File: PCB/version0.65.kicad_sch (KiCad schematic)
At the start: 142 parts, among them SW1 SW_SPDT, U1 SuperMini nRF52840

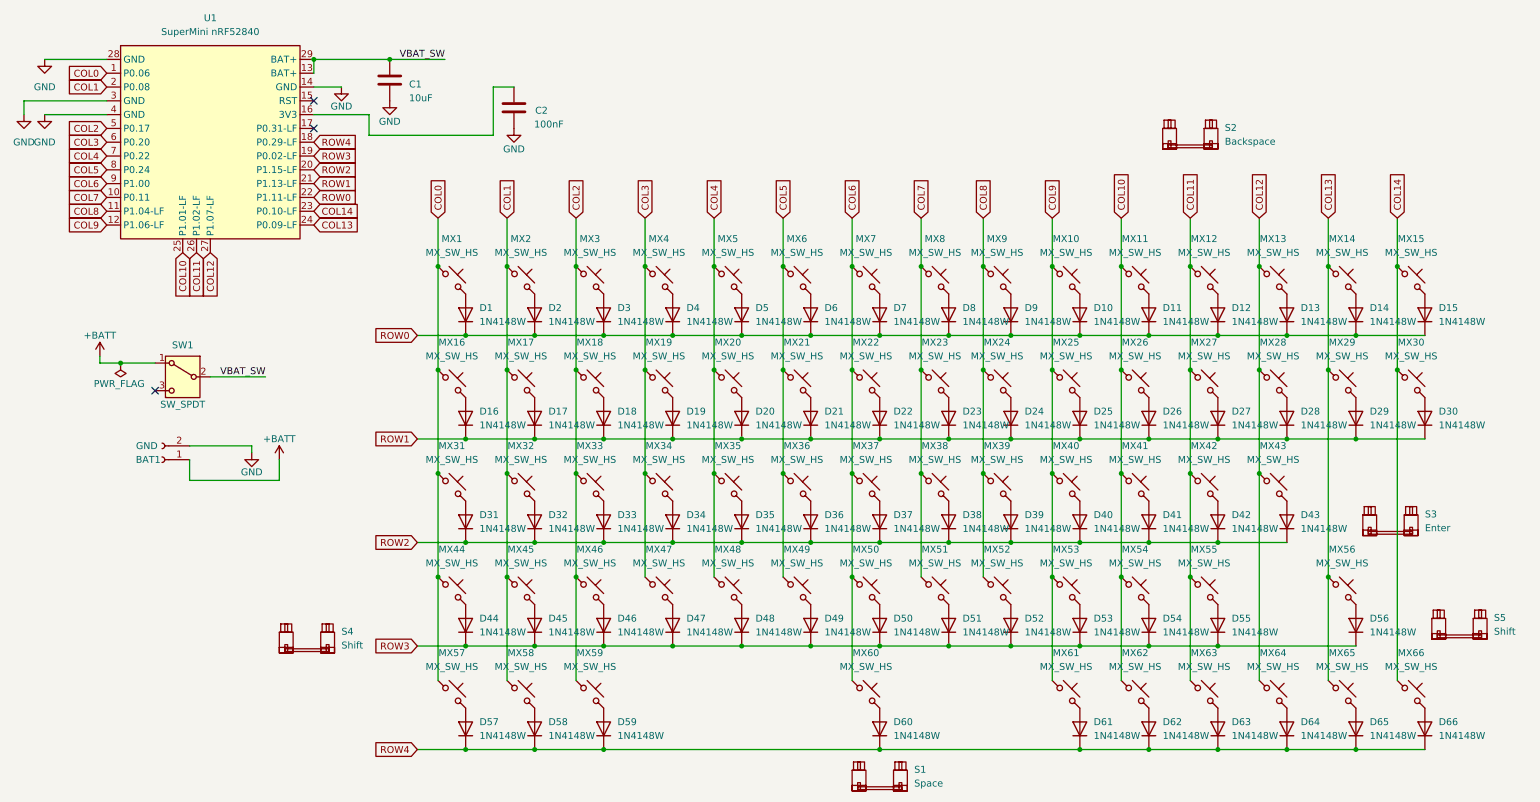
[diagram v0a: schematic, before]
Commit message: Updated PCB files
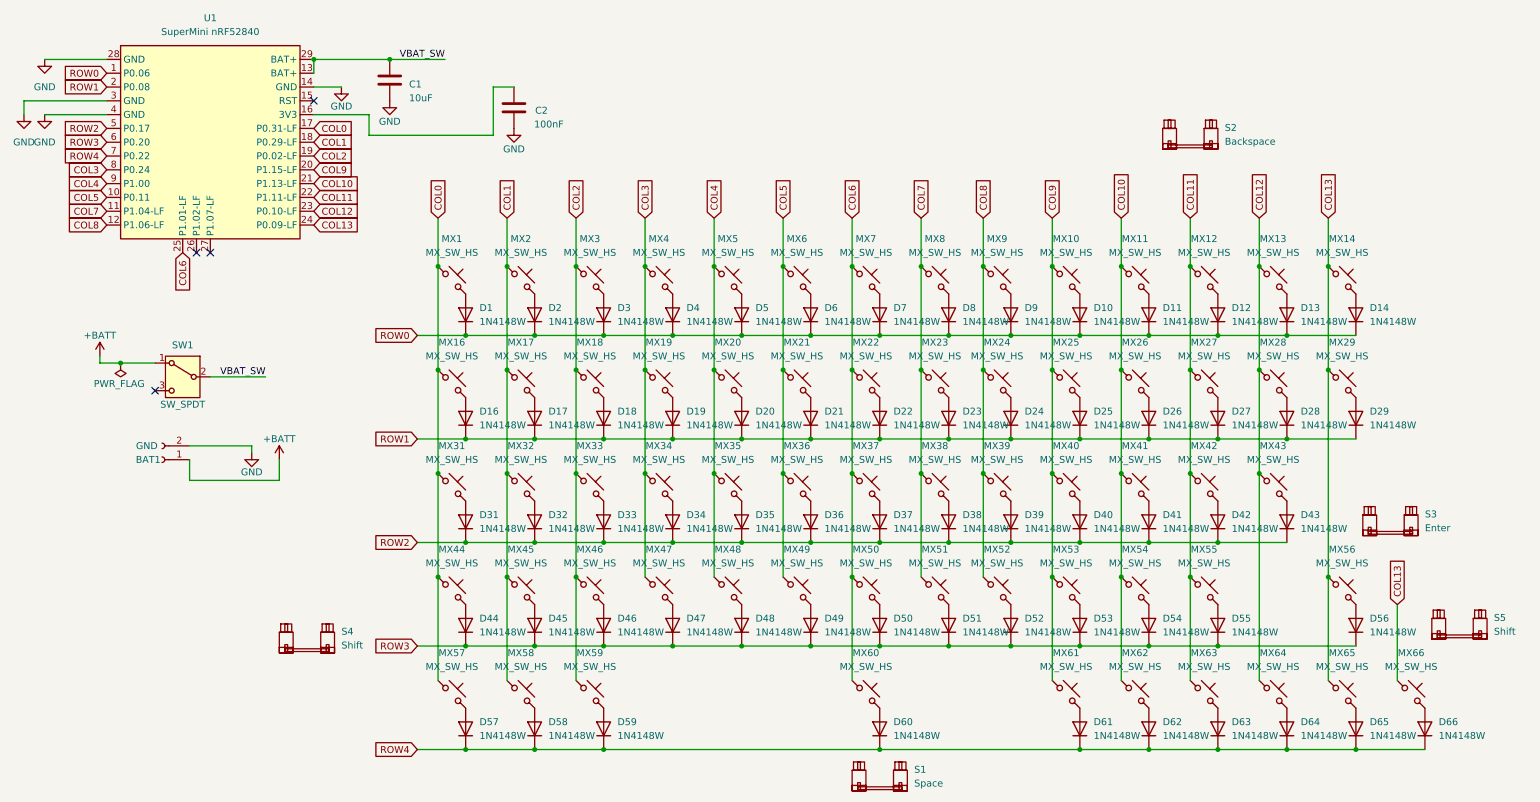
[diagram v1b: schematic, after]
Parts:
- removed D15, D30: 1N4148W, Diode_SMD:D_SOD-123, symbol Diode:1N4148W
- removed MX15, MX30: MX_SW_HS, PCM_marbastlib-mx:SW_MX_HS_KS-2P02B01-01_1u, symbol PCM_marbastlib-mx:MX_SW_HS_KS-2P02B01-01
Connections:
- net COL0: now also U1.17 (P0.31-LF); no longer U1.1 (P0.06)
- net COL1: now also U1.18 (P0.29-LF); no longer U1.2 (P0.08)
- net COL10: now also U1.21 (P1.13-LF); no longer U1.25 (P1.01-LF)
- net COL11: now also U1.22 (P1.11-LF); no longer U1.26 (P1.02-LF)
- net COL12: now also U1.23 (P0.10-LF); no longer U1.27 (P1.07-LF)
- net COL13: now also MX66.1
- net COL2: now also U1.19 (P0.02-LF); no longer U1.5 (P0.17)
- net COL3: now also U1.8 (P0.24); no longer U1.6 (P0.20)
- net COL4: now also U1.9 (P1.00); no longer U1.7 (P0.22)
- net COL5: now also U1.10 (P0.11); no longer U1.8 (P0.24)
- net COL6: now also U1.25 (P1.01-LF); no longer U1.9 (P1.00)
- net COL7: now also U1.11 (P1.04-LF); no longer U1.10 (P0.11)
- net COL8: now also U1.12 (P1.06-LF); no longer U1.11 (P1.04-LF)
- net COL9: now also U1.20 (P1.15-LF); no longer U1.12 (P1.06-LF)
- net ROW0: now also U1.1 (P0.06); no longer U1.22 (P1.11-LF)
- net ROW1: now also U1.2 (P0.08); no longer U1.21 (P1.13-LF)
- net ROW2: now also U1.5 (P0.17); no longer U1.20 (P1.15-LF)
- net ROW3: now also U1.6 (P0.20); no longer U1.19 (P0.02-LF)
- net ROW4: now also U1.7 (P0.22); no longer U1.18 (P0.29-LF)
- removed net COL14: MX66.1, U1.23 (P0.10-LF)
- no-connect marks 3 -> 4
